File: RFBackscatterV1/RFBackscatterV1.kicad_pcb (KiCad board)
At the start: 2 copper layers, 20.2 x 42.9 mm, 14 parts, among them J1 SMA-J-P-H-RA-TH1, U1 SIT1534AI-H4-DCC-00.001E

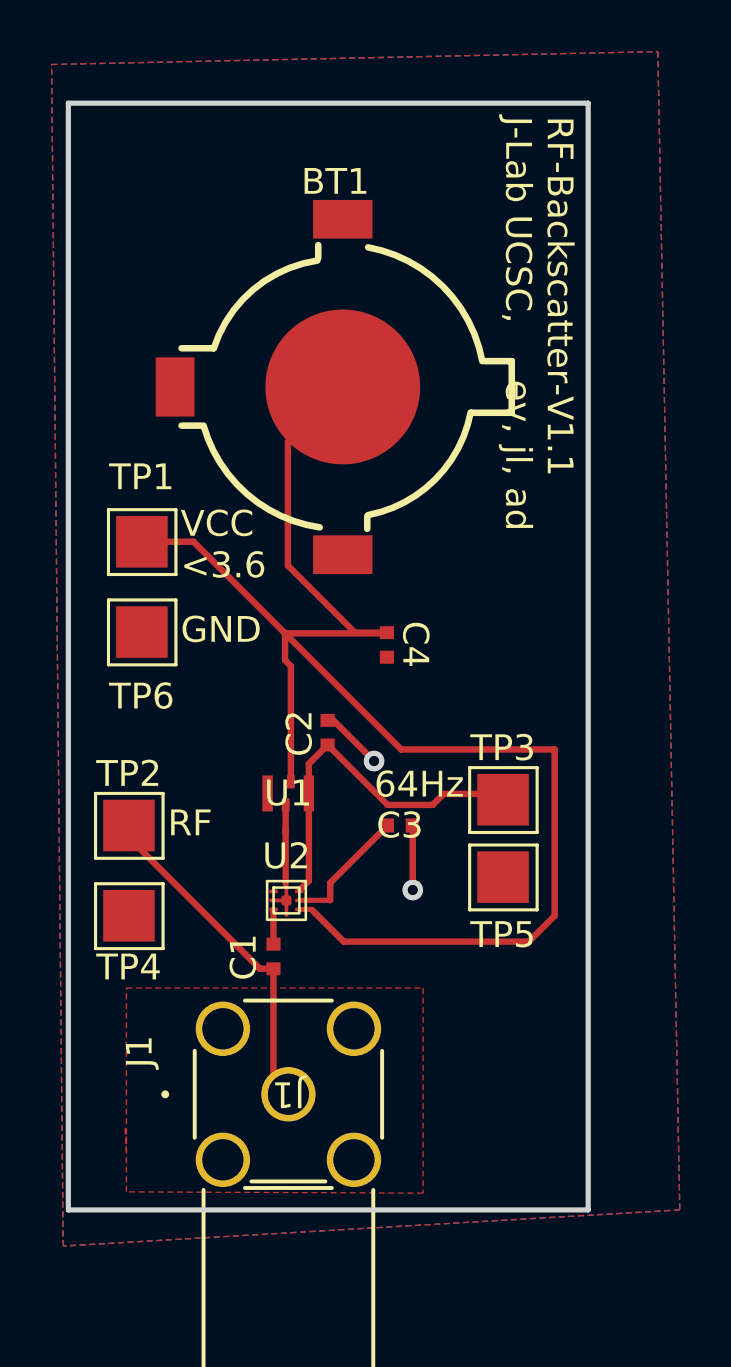
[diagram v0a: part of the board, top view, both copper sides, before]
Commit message: PCB updated
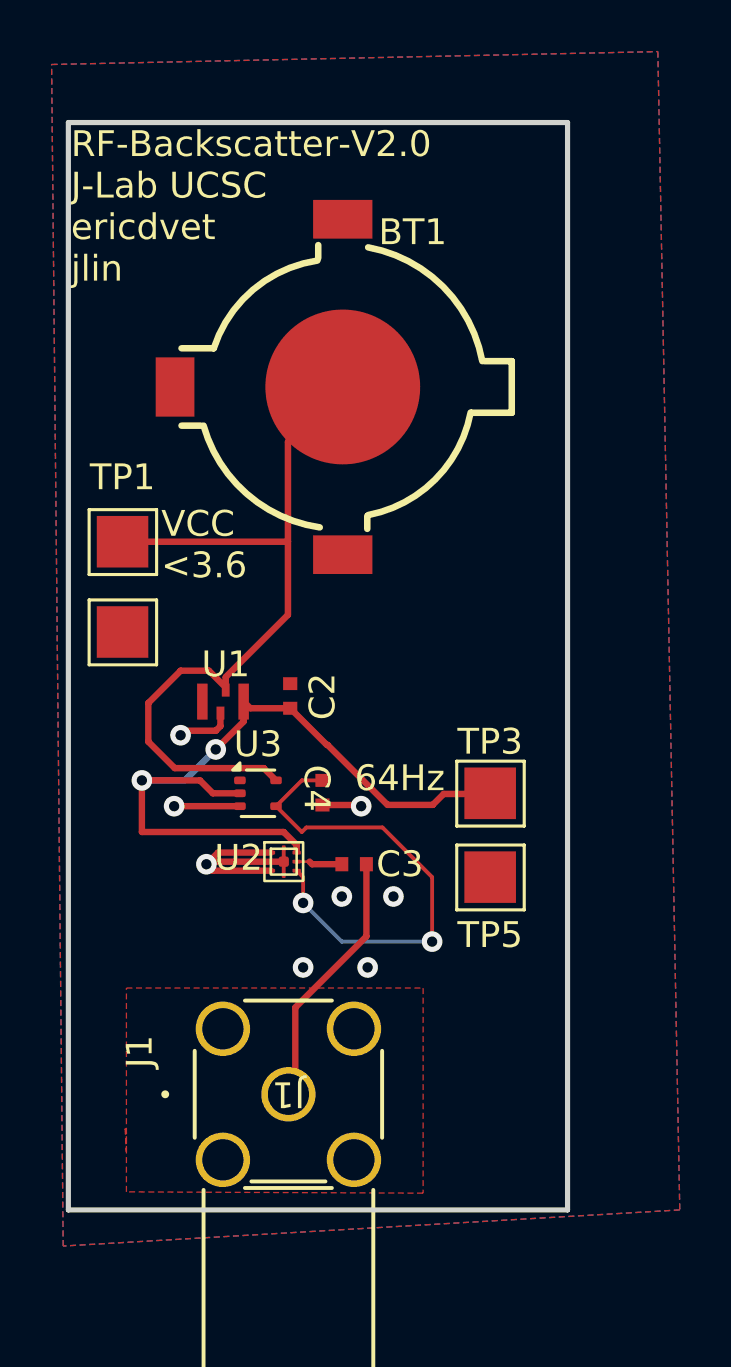
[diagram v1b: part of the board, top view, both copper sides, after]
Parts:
- removed C1: 100pF, WADARfootprints:CAPC10555_55N_KEM
- removed TP2: OUTPUT2, JLab_FP:EpicTestPointV1
- removed TP4: GND, JLab_FP:EpicTestPointV1
- added U3: 74LVC1GU04DRL, Package_TO_SOT_SMD:SOT-553, F.Cu at (169.0, 80.8)
- TP1: renamed from TP1 
- moved C4 6.25 mm to (171.5, 80.7)
- moved U1 4.36 mm to (167.6, 77.2)
- moved C3 2.32 mm to (172.7, 83.5)
- moved C2 2.03 mm to (170.2, 77.0)
- moved U2 1.51 mm to (170.0, 78.7)
- moved TP1 0.75 mm to (164.2, 73.7)
- moved TP6 0.75 mm to (164.2, 77.2)
- moved TP3 0.56 mm to (178.5, 83.5)
- moved TP5 0.50 mm to (178.5, 86.7)
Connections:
- C3 pad 2: GND -> Net-(C3-Pad2)
- C4 pad 1: +1V8 -> Net-(U2-VCTL2)
- J1 pad 1: Net-(C1-Pad2) -> Net-(C3-Pad2)
- U2 pad 1: unconnected-(U2-OUTPUT1-Pad1) -> GND
- U2 pad 3: Net-(U2-OUTPUT2) -> GND
- U2 pad 4: +1V8 -> Net-(U2-VCTL2)
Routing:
- net +1V8: track 59.2 -> 30.3 mm
- net Net-(U2-VCTL2): track 0.00 -> 19.0 mm, vias 0 -> 2
- net Net-(U1-CLK_Out): track 14.1 -> 30.1 mm, vias 0 -> 2
- net Net-(C1-Pad2): track 13.6 -> 0.00 mm
- net Net-(C3-Pad2): track 0.00 -> 10.6 mm
- net GND: track 8.09 -> 14.6 mm, vias 2 -> 8
- net Net-(U2-INPUT): track 4.92 -> 1.79 mm
- net Net-(U2-OUTPUT2): track 1.30 -> 0.00 mm
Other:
- board size 20.2 x 42.9 mm -> 19.3 x 42.2 mm
- board text added: "RF-Backscatter-V2.0 J-Lab UCSC ericdvet jlin"
- board text removed: "GND"
- board text removed: "RF"
- board text removed: "RF-Backscatter-V1.1 J-Lab UCSC, ev, jl, ad"

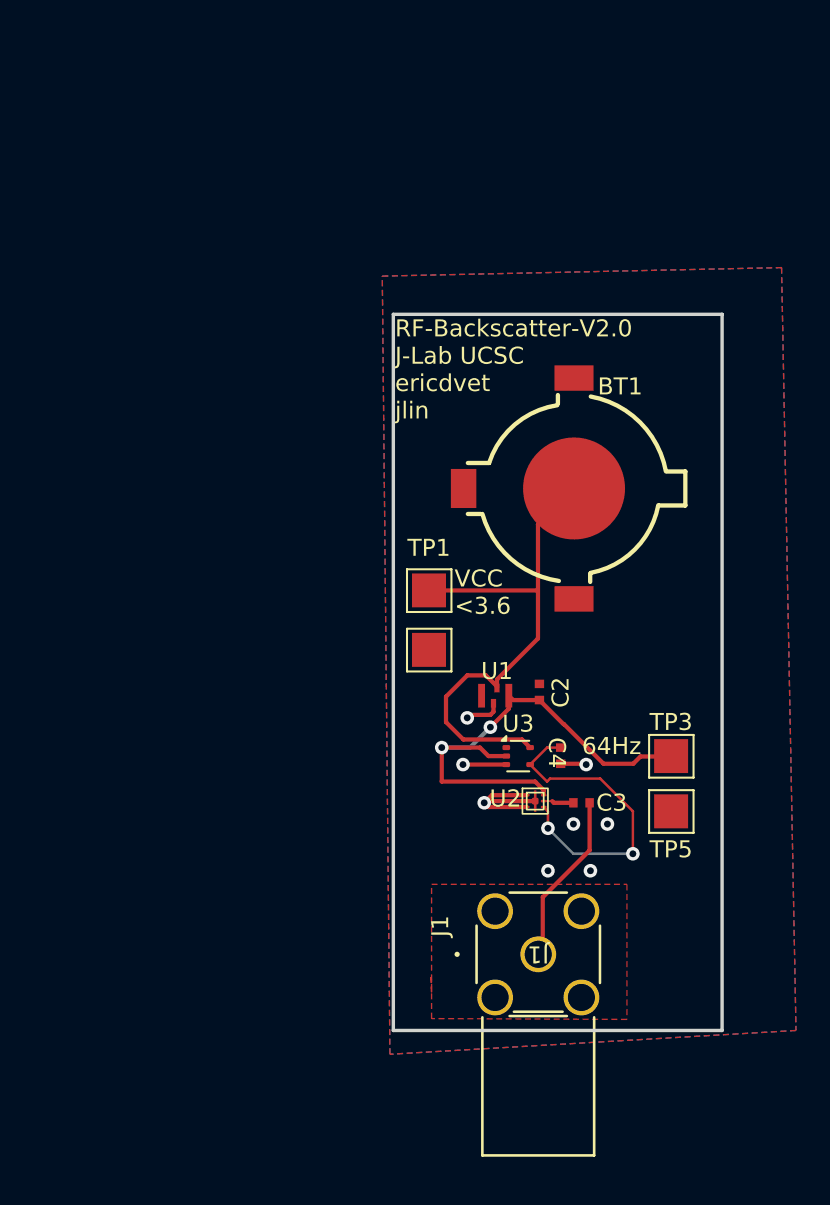
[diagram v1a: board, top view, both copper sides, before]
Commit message: alexandre's advice pt2
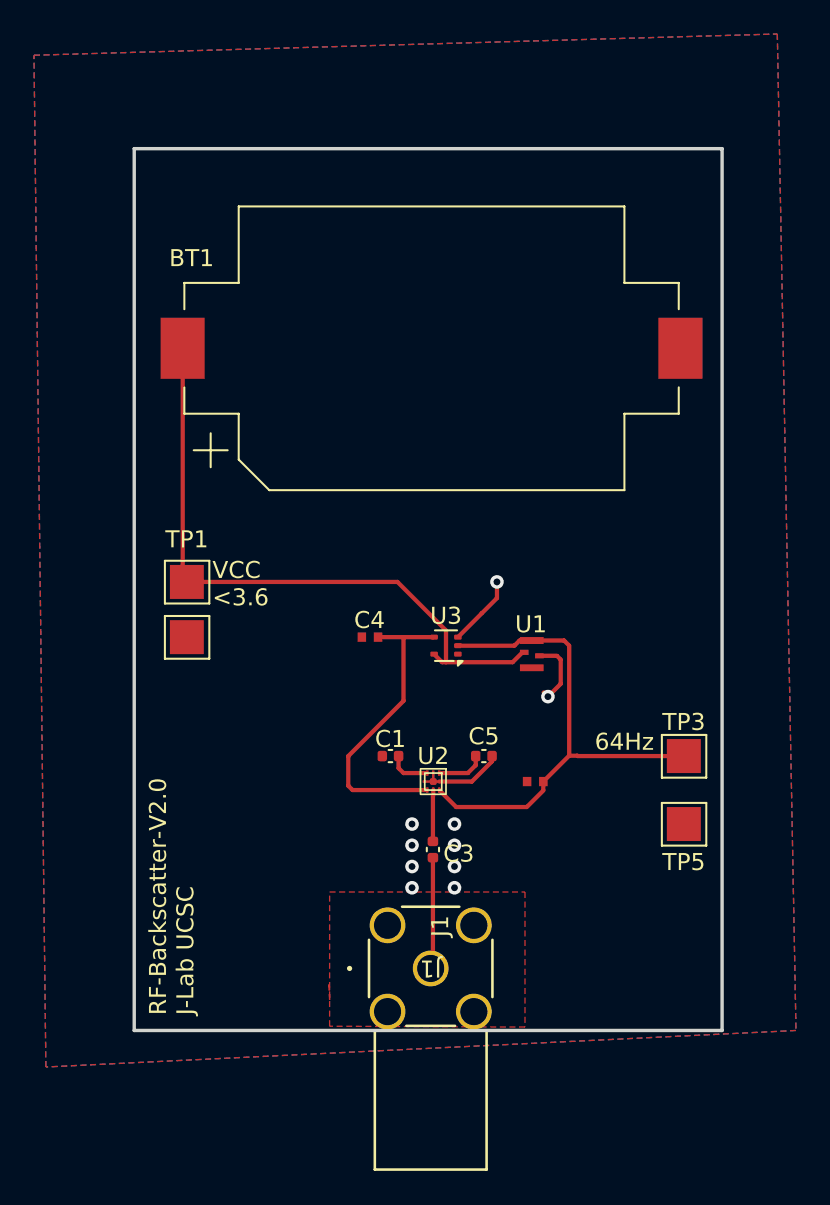
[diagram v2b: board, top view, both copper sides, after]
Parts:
- added C1: 10nF, Capacitor_SMD:C_0402_1005Metric, F.Cu at (161.5, 80.8)
- added C5: 10nF, Capacitor_SMD:C_0402_1005Metric, F.Cu at (167.0, 80.8)
- BT1: footprint WADARfootprints:BAT-SMD_MY-LR44-02 -> Battery:BatteryHolder_Keystone_1060_1x2032
- C3: value 100pF -> 10nF; footprint JLab_FP:CAPC10555_55N_KEM -> Capacitor_SMD:C_0402_1005Metric
- moved TP6 14.3 mm to (150.0, 76.5)
- moved TP1 14.3 mm to (150.0, 73.2)
- moved C4 13.2 mm to (160.3, 73.8), turned to 180 degrees
- moved BT1 9.72 mm to (163.9, 56.8)
- moved C3 9.17 mm to (164.0, 86.2), turned to -90 degrees
- moved U3 7.77 mm to (164.8, 74.2), turned to 180 degrees
- moved J1 6.38 mm to (163.8, 93.2)
- moved C2 5.28 mm to (170.0, 82.2), turned to 180 degrees
- moved U2 3.81 mm to (168.8, 82.2), turned to -90 degrees
- moved U1 3.26 mm to (169.8, 74.8), turned to 90 degrees
- moved TP5 1.06 mm to (179.2, 87.5)
- moved TP3 0.75 mm to (179.2, 83.5)
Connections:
- net +1V8 renamed 3V0
- U2 pad 1: GND -> Net-(U2-OUTPUT1)
- U2 pad 3: GND -> Net-(U2-OUTPUT2)
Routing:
- net 3V0: track 30.3 -> 37.9 mm
- net Net-(C3-Pad2): track 10.6 -> 6.76 mm
- net Net-(U2-OUTPUT1): track 0.00 -> 2.83 mm
- net Net-(U2-OUTPUT2): track 0.00 -> 2.47 mm
- net GND: track 14.6 -> 12.3 mm, vias 8 -> 10
- net Net-(U2-INPUT): track 1.79 -> 3.03 mm
- net Net-(U2-VCTL2): track 19.0 -> 18.1 mm, vias 2 -> 0
- net Net-(U1-CLK_Out): track 30.1 -> 29.6 mm, vias 2 -> 0
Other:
- board size 19.3 x 42.2 mm -> 34.6 x 51.9 mm
- board text added: "RF-Backscatter-V2.0 J-Lab UCSC"
- board text removed: "RF-Backscatter-V2.0 J-Lab UCSC ericdvet jlin"
